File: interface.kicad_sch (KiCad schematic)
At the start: 15 parts, among them J10 Conn_01x04, J12 Conn_01x08, J13 Conn_01x08, J14 Conn_01x08, J15 Conn_01x08, J16 Conn_01x16, J17 Conn_01x08, J18 Conn_01x06, J3 JTAG, J4 Conn_01x08, J5 Conn_01x16, J6 Conn_01x04, J7 Conn_01x08, J8 Conn_01x06, J9 Conn_01x08

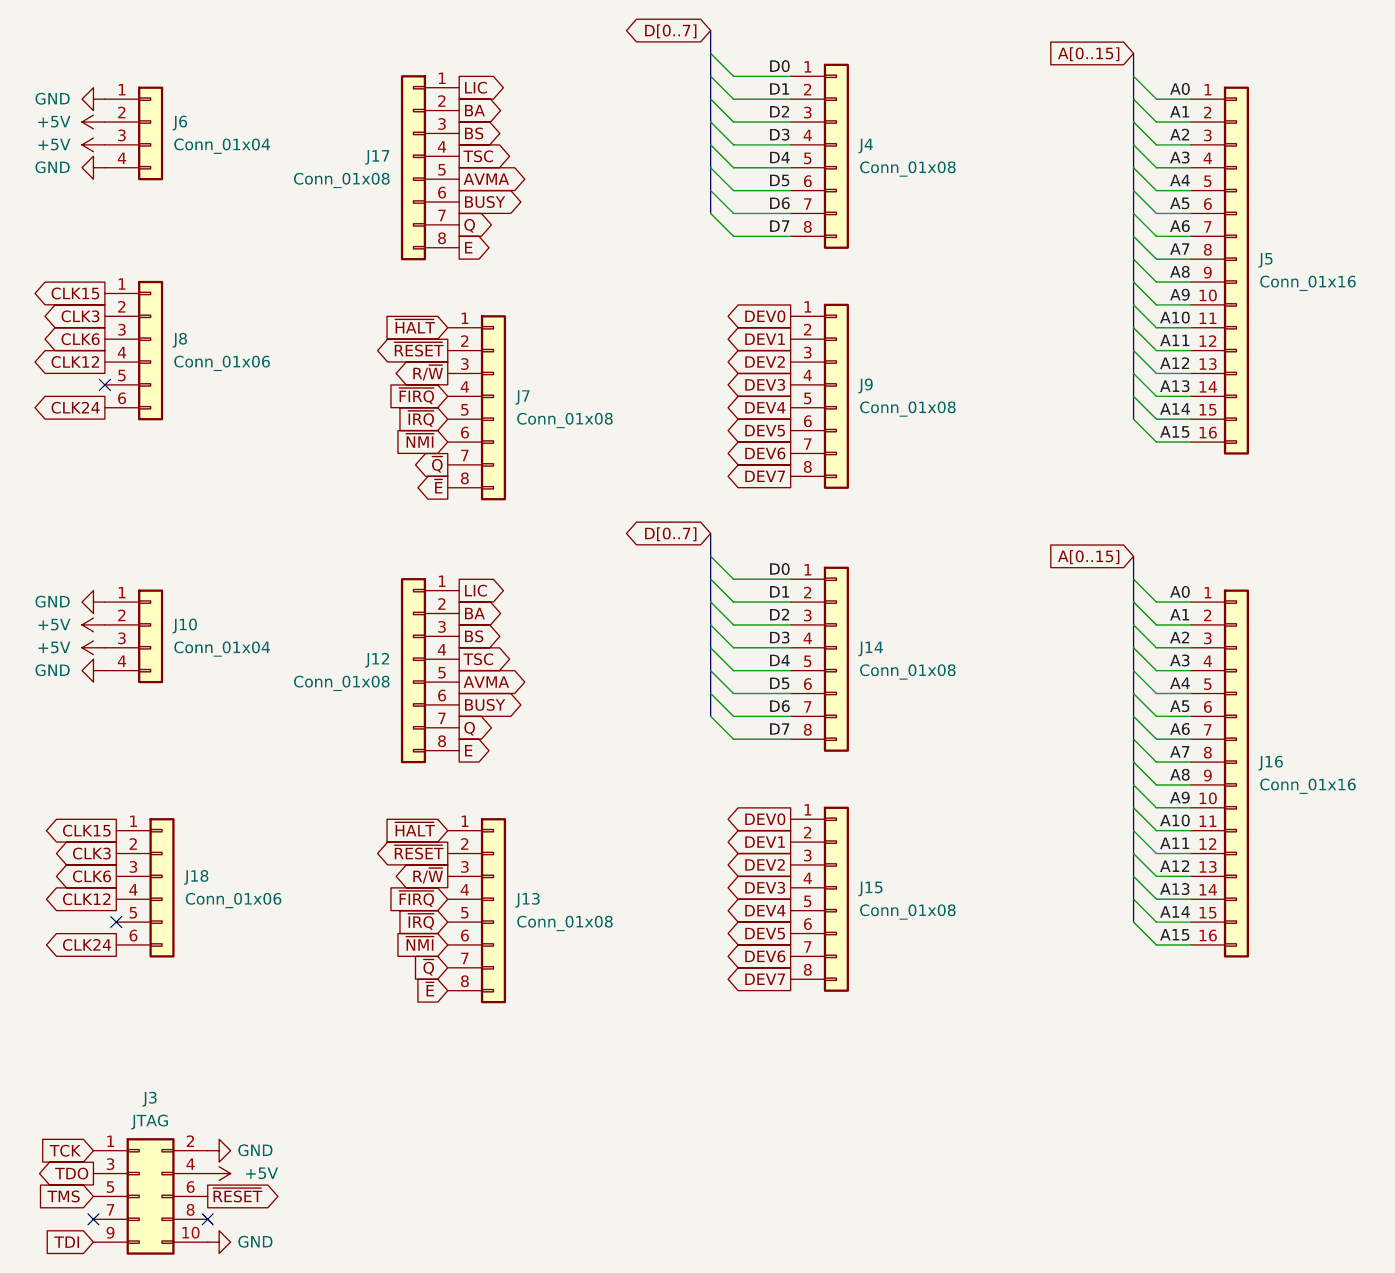
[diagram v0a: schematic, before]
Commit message: convert to dragon
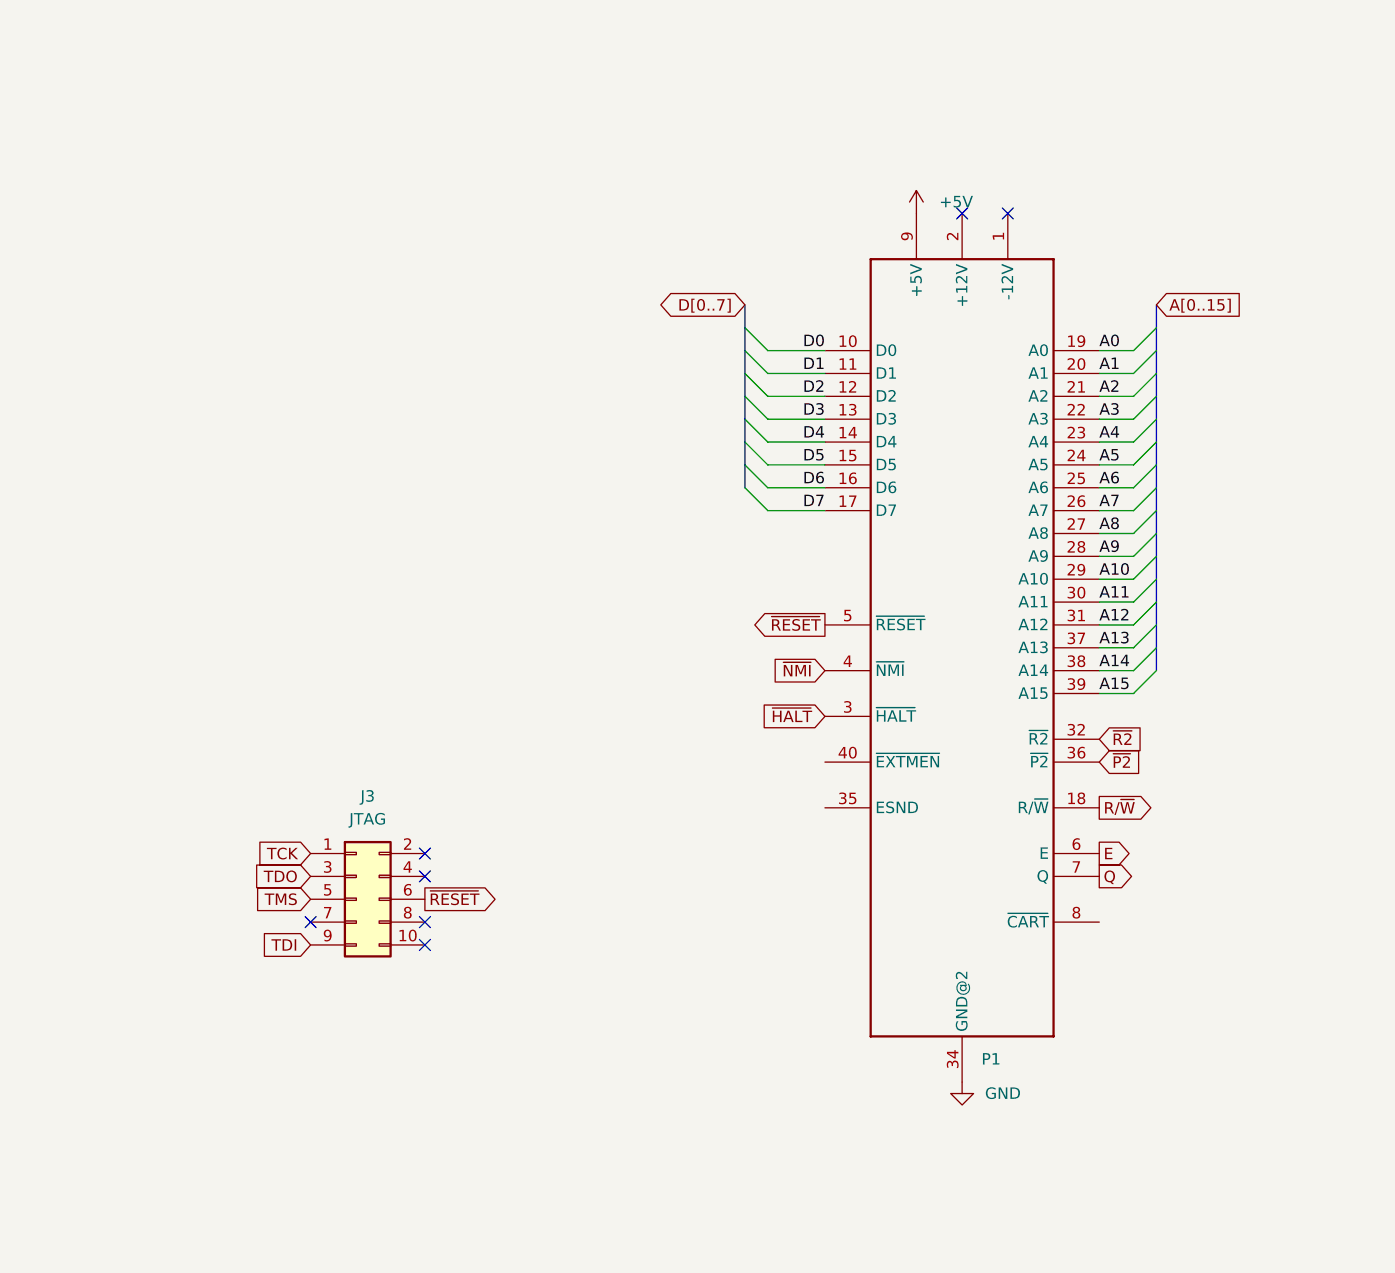
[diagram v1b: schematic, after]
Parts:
- removed J10, J6: Conn_01x04, Connector_PinHeader_2.54mm:PinHeader_1x04_P2.54mm_Vertical, symbol Connector_Generic:Conn_01x04
- removed J12, J13, J14, J15, J17, J4, J7, J9: Conn_01x08, Connector_PinHeader_2.54mm:PinHeader_1x08_P2.54mm_Vertical, symbol Connector_Generic:Conn_01x08
- removed J16, J5: Conn_01x16, Connector_PinHeader_2.54mm:PinHeader_1x16_P2.54mm_Vertical, symbol Connector_Generic:Conn_01x16
- removed J18, J8: Conn_01x06, Connector_PinHeader_2.54mm:PinHeader_1x06_P2.54mm_Vertical, symbol Connector_Generic:Conn_01x06
- added P1: ~, Library:CartridgeEdge, symbol Library:CartridgeEdge
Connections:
- net +5V: now also P1.9 (+5V); no longer J3.4 (Pin_4)
- net A0: now also P1.19 (A0)
- net A1: now also P1.20 (A1)
- net A10: now also P1.29 (A10)
- net A11: now also P1.30 (A11)
- net A12: now also P1.31 (A12)
- net A13: now also P1.37 (A13)
- net A14: now also P1.38 (A14)
- net A15: now also P1.39 (A15)
- net A2: now also P1.21 (A2)
- net A3: now also P1.22 (A3)
- net A4: now also P1.23 (A4)
- net A5: now also P1.24 (A5)
- net A6: now also P1.25 (A6)
- net A7: now also P1.26 (A7)
- net A8: now also P1.27 (A8)
- net A9: now also P1.28 (A9)
- net D0: now also P1.10 (D0)
- net D1: now also P1.11 (D1)
- net D2: now also P1.12 (D2)
- net D3: now also P1.13 (D3)
- net D4: now also P1.14 (D4)
- net D5: now also P1.15 (D5)
- net D6: now also P1.16 (D6)
- net D7: now also P1.17 (D7)
- net E: now also P1.6 (E)
- net GND: now also P1.33 (GND@1), P1.34 (GND@2); no longer J3.10 (Pin_10), J3.2 (Pin_2)
- net Q: now also P1.7 (Q)
- net R/~{W}: now also P1.18 (R/~{W})
- net ~{HALT}: now also P1.3 (~{HALT})
- net ~{NMI}: now also P1.4 (~{NMI})
- net ~{RESET}: now also P1.5 (~{RESET})
- new net ~{P2}: P1.36 (~{P2})
- new net ~{R2}: P1.32 (~{R2})
- no-connect marks 4 -> 7

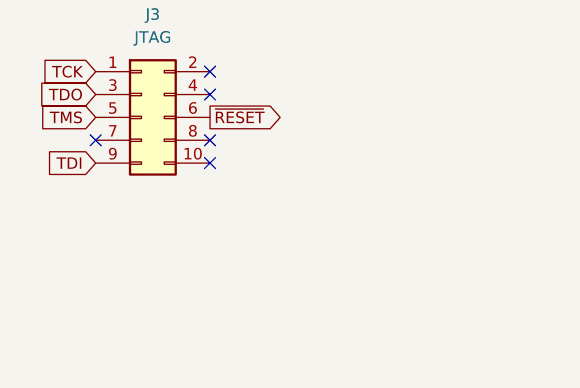
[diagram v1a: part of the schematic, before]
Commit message: refresh bom
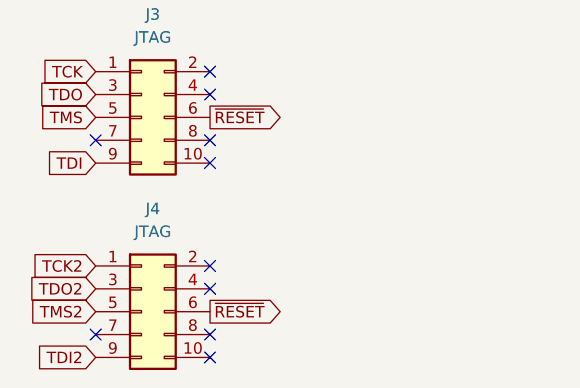
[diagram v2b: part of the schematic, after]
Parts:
- added J4: JTAG, Connector_PinHeader_2.54mm:PinHeader_2x05_P2.54mm_Vertical, symbol Connector_Generic:Conn_02x05_Odd_Even
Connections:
- net ~{RESET}: now also J4.6 (Pin_6)
- new net TCK2: J4.1 (Pin_1)
- new net TDI2: J4.9 (Pin_9)
- new net TDO2: J4.3 (Pin_3)
- new net TMS2: J4.5 (Pin_5)
- no-connect marks 7 -> 12
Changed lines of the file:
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@@
 	(paper "A4")
 	(no_connect
+		(at 67.31 142.24)
+	)
+	(no_connect
 		(at 67.31 113.03)
 	)
@@
 	)
 	(no_connect
+		(at 67.31 134.62)
+	)
+	(no_connect
+		(at 54.61 139.7)
+	)
+	(no_connect
 		(at 132.08 39.37)
 	)
@@
 	)
 	(no_connect
+		(at 67.31 139.7)
+	)
+	(no_connect
 		(at 67.31 118.11)
 	)
 	(no_connect
 		(at 127 39.37)
+	)
+	(no_connect
+		(at 67.31 132.08)
 	)
 	(bus_entry
@@
 	(global_label "~{RESET}"
 		(shape output)
+		(at 67.31 137.16 0)
+		(fields_autoplaced yes)
+		(effects
+			(font
+				(size 1.27 1.27)
+			)
+			(justify left)
+		)
+		(property "Intersheetrefs" "${INTERSHEET_REFS}"
+			(at 76.0403 137.16 0)
+			(effects
+				(font
+					(size 1.27 1.27)
+				)
+				(justify left)
+				(hide yes)
+			)
+		)
+	)
+	(global_label "~{RESET}"
+		(shape output)
 		(at 111.76 85.09 180)
 		(fields_autoplaced yes)
@@
 		)
 	)
+	(global_label "TMS2"
+		(shape input)
+		(at 54.61 137.16 180)
+		(fields_autoplaced yes)
+		(effects
+			(font
+				(size 1.27 1.27)
+			)
+			(justify right)
+		)
+		(property "Intersheetrefs" "${INTERSHEET_REFS}"
+			(at 46.7868 137.16 0)
+			(effects
+				(font
+					(size 1.27 1.27)
+				)
+				(justify right)
+				(hide yes)
+			)
+		)
+	)
 	(global_label "TMS"
 		(shape input)
@@
 		)
 	)
+	(global_label "TDI2"
+		(shape input)
+		(at 54.61 142.24 180)
+		(fields_autoplaced yes)
+		(effects
+			(font
+				(size 1.27 1.27)
+			)
+			(justify right)
+		)
+		(property "Intersheetrefs" "${INTERSHEET_REFS}"
+			(at 48.7824 142.24 0)
+			(effects
+				(font
+					(size 1.27 1.27)
+				)
+				(justify right)
+				(hide yes)
+			)
+		)
+	)
+	(global_label "TDO2"
+		(shape input)
+		(at 54.61 134.62 180)
+		(fields_autoplaced yes)
+		(effects
+			(font
+				(size 1.27 1.27)
+			)
+			(justify right)
+		)
+		(property "Intersheetrefs" "${INTERSHEET_REFS}"
+			(at 48.0567 134.62 0)
+			(effects
+				(font
+					(size 1.27 1.27)
+				)
+				(justify right)
+				(hide yes)
+			)
+		)
+	)
 	(global_label "~{HALT}"
 		(shape input)
@@
 				)
 				(justify left)
+				(hide yes)
+			)
+		)
+	)
+	(global_label "TCK2"
+		(shape input)
+		(at 54.61 132.08 180)
+		(fields_autoplaced yes)
+		(effects
+			(font
+				(size 1.27 1.27)
+			)
+			(justify right)
+		)
+		(property "Intersheetrefs" "${INTERSHEET_REFS}"
+			(at 46.9077 132.08 0)
+			(effects
+				(font
+					(size 1.27 1.27)
+				)
+				(justify right)
 				(hide yes)
 			)
@@
 					(unit 1)
 				)
+			)
+		)
+	)
+	(symbol
+		(lib_id "Connector_Generic:Conn_02x05_Odd_Even")
+		(at 59.69 137.16 0)
+		(unit 1)
+		(exclude_from_sim no)
+		(in_bom yes)
+		(on_board yes)
+		(dnp no)
+		(fields_autoplaced yes)
+		(property "Reference" "J4"
+			(at 60.96 125.73 0)
+			(effects
+				(font
+					(size 1.27 1.27)
+				)
+			)
+		)
+		(property "Value" "JTAG"
+			(at 60.96 128.27 0)
+			(effects
+				(font
+					(size 1.27 1.27)
+				)
+			)
+		)
+		(property "Footprint" "Connector_PinHeader_2.54mm:PinHeader_2x05_P2.54mm_Vertical"
+			(at 59.69 137.16 0)
+			(effects
+				(font
+					(size 1.27 1.27)
+				)
+				(hide yes)
+			)
+		)
+		(property "Datasheet" "~"
+			(at 59.69 137.16 0)
+			(effects
+				(font
+					(size 1.27 1.27)
+				)
+				(hide yes)
+			)
+		)
+		(property "Description" "Generic connector, double row, 02x05, odd/even pin numbering scheme (row 1 odd numbers, row 2 even numbers), script generated (kicad-library-utils/schlib/autogen/connector/)"
+			(at 59.69 137.16 0)
+			(effects
+				(font
+					(size 1.27 1.27)
+				)
+				(hide yes)
+			)
+		)
+		(pin "4"
+		)
+		(pin "5"
+		)
+		(pin "9"
+		)
+		(pin "7"
+		)
+		(pin "1"
+		)
+		(pin "3"
+		)
+		(pin "2"
+		)
+		(pin "8"
+		)
+		(pin "6"
+		)
+		(pin "10"
+		)
+		(instances
+			(project "SBC6809System2Video"
+				(path "/78b9551b-1c10-4835-8047-f82ce94e7825/0fadc3d1-9644-458b-8592-35be0cb0a9ca"
+					(reference "J4")
+					(unit 1)
+				)
